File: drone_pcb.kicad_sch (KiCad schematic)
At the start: 35 parts, among them J1 HappyModel EP1, J10 M4_NEG, J2 BATT, J3 M1_NEG, J4 M1_POS, J5 M2_POS, J6 M2_NEG, J7 M3_POS, J8 M3_NEG, J9 M4_POS, Q1 AO3400A, Q2 AO3400A, Q3 AO3400A, Q4 AO3400A, U1 OC09600, U2 AP2112K-3.3

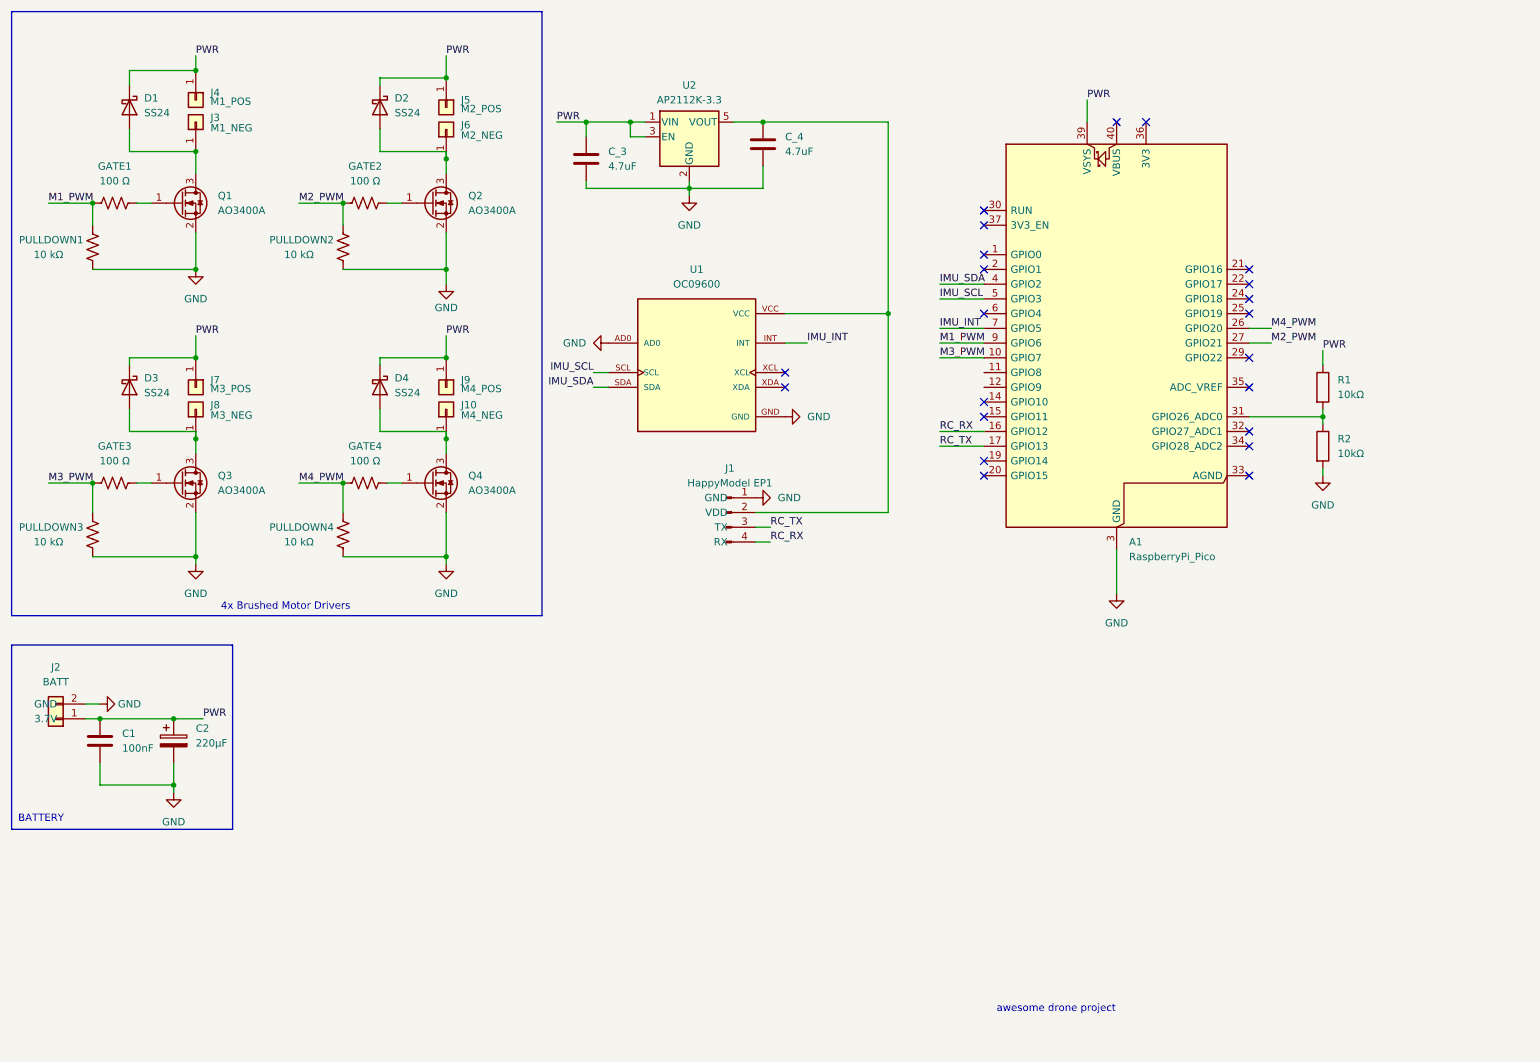
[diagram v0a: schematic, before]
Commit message: final draft i think
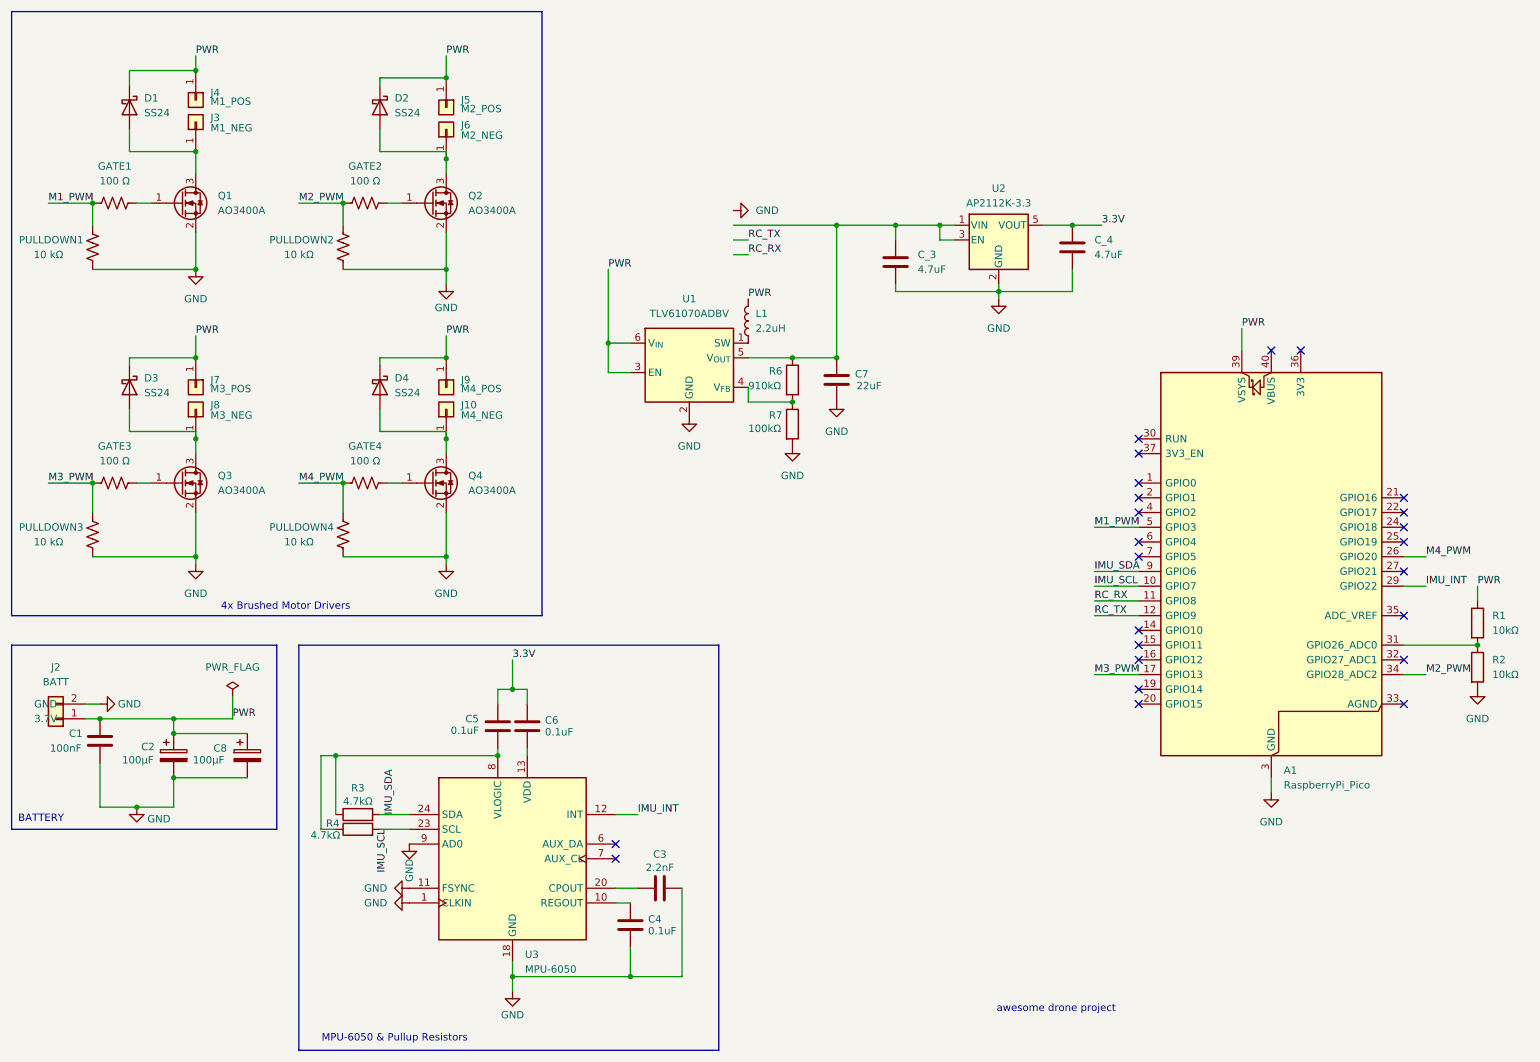
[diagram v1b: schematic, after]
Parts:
- removed J1: HappyModel EP1, Connector_PinHeader_2.54mm:PinHeader_1x04_P2.54mm_Vertical, symbol Connector:Conn_01x04_Pin
- removed U1: OC09600, OC09600:MODULE_OC09600, symbol OC09600:OC09600
- added C3: 2.2nF, Capacitor_SMD:C_0805_2012Metric, symbol Device:C
- added C4, C5, C6: 0.1uF, Capacitor_SMD:C_0805_2012Metric, symbol Device:C
- added C7: 22uF, Capacitor_SMD:C_0805_2012Metric, symbol Device:C
- added C8: 100µF, Capacitor_SMD:C_1206_3216Metric, symbol Device:C_Polarized
- added L1: 2.2uH, Inductor_SMD:L_1008_2520Metric, symbol Device:L
- added R3, R4: 4.7kΩ, Resistor_SMD:R_0805_2012Metric, symbol Device:R
- added R6: 910kΩ, Resistor_SMD:R_0805_2012Metric, symbol Device:R
- added R7: 100kΩ, Resistor_SMD:R_0805_2012Metric, symbol Device:R
- added U1: TLV61070ADBV, Package_TO_SOT_SMD:SOT-23-6, symbol Regulator_Switching:TLV61070ADBV
- added U3: MPU-6050, Sensor_Motion:InvenSense_QFN-24_4x4mm_P0.5mm, symbol Sensor_Motion:MPU-6050
- C2: value 220µF -> 100µF; footprint Capacitor_SMD:C_1210_3225Metric -> Capacitor_SMD:C_1206_3216Metric
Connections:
- net GND: now also C3.2, C4.2, C7.2, C8.2, R7.2, U1.2 (GND), U3.1 (CLKIN), U3.11 (FSYNC), U3.18 (GND), U3.9 (AD0)
- net IMU_INT: now also A1.29 (GPIO22), U3.12 (INT); no longer A1.7 (GPIO5)
- net IMU_SCL: now also A1.10 (GPIO7), R4.2, U3.23 (SCL); no longer A1.5 (GPIO3)
- net IMU_SDA: now also A1.9 (GPIO6), R3.2, U3.24 (SDA); no longer A1.4 (GPIO2)
- net M1_PWM: now also A1.5 (GPIO3); no longer A1.9 (GPIO6)
- net M2_PWM: now also A1.34 (GPIO28_ADC2); no longer A1.27 (GPIO21)
- net M3_PWM: now also A1.17 (GPIO13); no longer A1.10 (GPIO7)
- net PWR: now also C8.1, L1.2, U1.3 (EN), U1.6 (V_{IN}); no longer C_3.1, U2.1 (VIN), U2.3 (EN)
- net RC_RX: now also A1.11 (GPIO8); no longer A1.16 (GPIO12)
- net RC_TX: now also A1.12 (GPIO9); no longer A1.17 (GPIO13)
- net 3.3V: now reaches C_4.1, U2.5 (VOUT)
- net 3.3V: now also C5.1, C6.1
- new net: C4.1, U3.10 (REGOUT)
- new net: L1.1, U1.1 (SW)
- new net: R6.2, R7.1, U1.4 (V_{FB})
- new net: C7.1, C_3.1, R6.1, U1.5 (V_{OUT}), U2.1 (VIN), U2.3 (EN)
- new net: C6.2, U3.13 (VDD)
- new net: C3.1, U3.20 (CPOUT)
- new net: C5.2, R3.1, R4.1, U3.8 (VLOGIC)
- no-connect marks 22 -> 24
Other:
- note added: "MPU-6050 & Pullup Resistors"
- moved on the sheet: A1, C2, C_3, C_4, R1, R2, U2
